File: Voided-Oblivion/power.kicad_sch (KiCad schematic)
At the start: 132 parts, among them Q1 AO3401, Q10 BC847B, Q11 BC847B, Q13 NCE4009S, Q14 NCE4009S, Q2 AO4407A, Q3 BC857, Q4 AO4407A, Q5 AO4407A, Q6 AO4407A, Q7 AO4407A, Q8 BC847B, Q9 BC847B, U10 TLV431BQDBZR, U11 LM2903, U12 AP2171WG-7, U13 TPD2E2U06DRL, U14 TPD2E2U06DRL, U15 LM66100DCKT, U16 AP2171WG-7, U17 LM74700QDDF, U18 LM74700QDDF, U2 TS3USB30ERSWR, U5 TPS54302, U6 TPS54302, U7 TLV76733DRVR, U9 LM66100DCKT

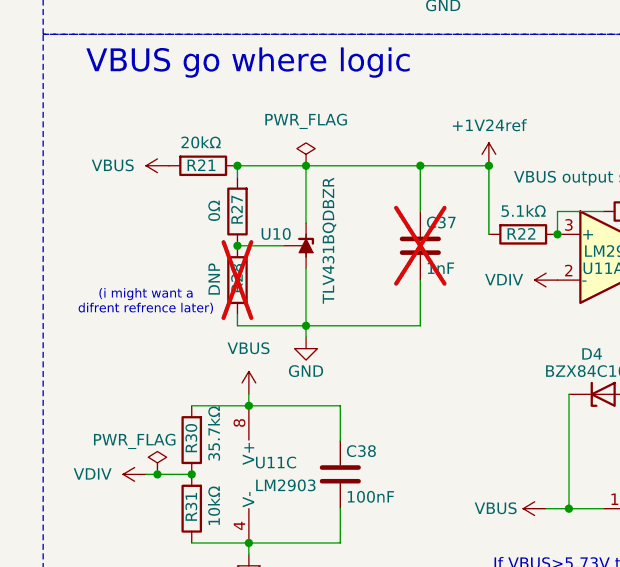
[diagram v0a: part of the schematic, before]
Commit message: production files i think.com
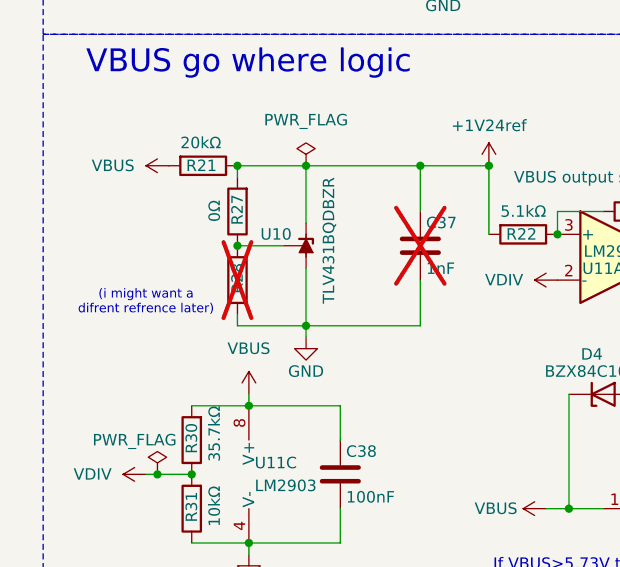
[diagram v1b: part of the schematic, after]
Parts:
- R28: value DNP -> (none); now left out of the parts list
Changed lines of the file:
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@@
 		(body_style 1)
 		(exclude_from_sim no)
-		(in_bom yes)
+		(in_bom no)
 		(on_board yes)
 		(in_pos_files no)
@@
 			)
 		)
-		(property "Value" "DNP"
+		(property "Value" ""
 			(at 35.56 175.895 90)
 			(show_name no)
@@
 		(in_bom no)
 		(on_board yes)
-		(in_pos_files yes)
+		(in_pos_files no)
 		(dnp yes)
 		(property "Reference" "C37"
